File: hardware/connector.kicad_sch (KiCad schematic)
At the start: 2 parts, among them J1 AXK5F20347YG, J2 AXK5F20347YG

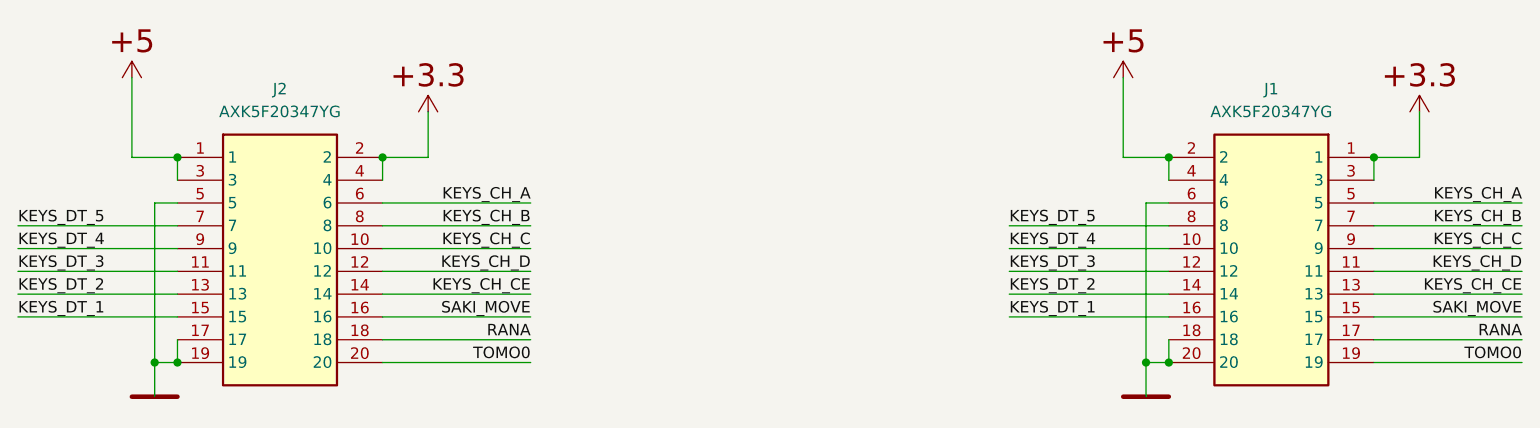
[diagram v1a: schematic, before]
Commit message: :sparkles: assembly all the part!
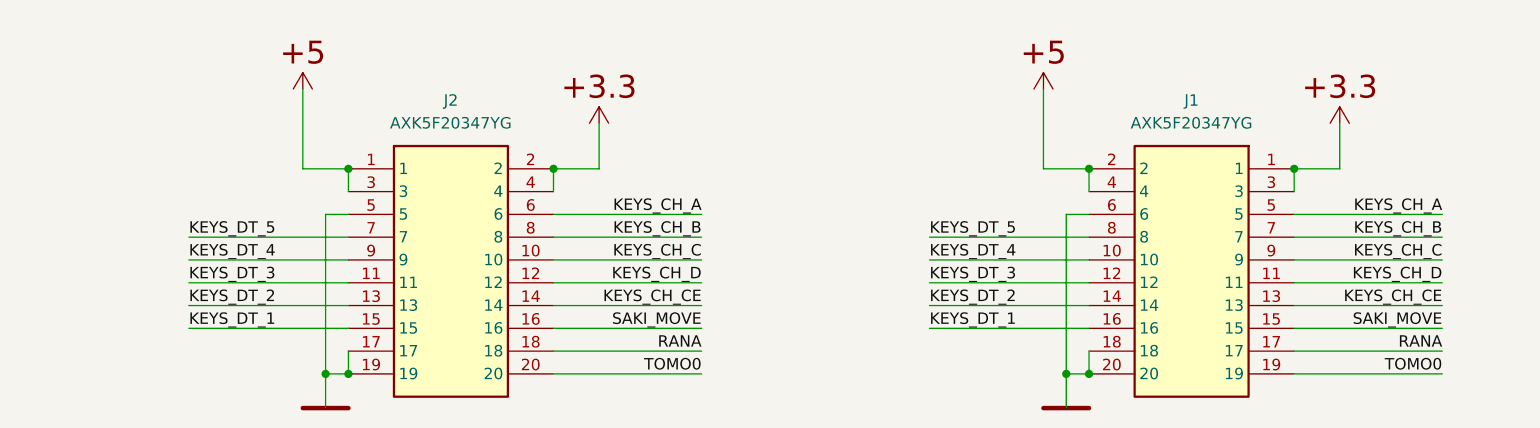
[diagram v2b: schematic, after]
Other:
- moved on the sheet: J1, J2
